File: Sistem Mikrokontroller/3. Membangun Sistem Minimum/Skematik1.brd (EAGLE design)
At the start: 59.4 x 57.1 mm, 20 parts, among them IC2 78L05Z, J1 DCJ0202, U1 328P

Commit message: update
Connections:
- removed net N$37: C3.2, C7.-, S2.2
- net GND: now also C3.2, C7.-, S2.2
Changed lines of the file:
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@@
 <contactref element="JP5" pad="3"/>
 <contactref element="JP5" pad="2"/>
-<wire x1="55.88" y1="41.91" x2="53.34" y2="52.07" width="0" layer="19" extent="1-1"/>
+<contactref element="C3" pad="2"/>
+<contactref element="C7" pad="-"/>
+<contactref element="S2" pad="2"/>
+<wire x1="55.88" y1="41.91" x2="68.58" y2="39.37" width="0" layer="19" extent="1-1"/>
 <wire x1="52.07" y1="40.64" x2="55.88" y2="41.91" width="0" layer="19" extent="16-16"/>
 <wire x1="41.275" y1="34.925" x2="50.8" y2="34.925" width="0" layer="19" extent="16-16"/>
 <wire x1="36.83" y1="27.94" x2="41.275" y2="34.925" width="0" layer="19" extent="16-16"/>
+<wire x1="53.34" y1="52.07" x2="55.88" y2="41.91" width="0" layer="19" extent="1-1"/>
 <wire x1="13.69" y1="22.86" x2="36.83" y2="27.94" width="0" layer="19" extent="1-1"/>
 <wire x1="8.89" y1="19.86" x2="13.69" y2="22.86" width="0" layer="19" extent="1-1"/>
@@
 <wire x1="17.78" y1="1.27" x2="15.24" y2="1.27" width="0" layer="19" extent="1-1"/>
 <wire x1="10.16" y1="-17.78" x2="10.16" y2="1.27" width="0" layer="19" extent="1-1"/>
-<wire x1="8.89" y1="-48.26" x2="10.16" y2="-17.78" width="0" layer="19" extent="1-1"/>
+<wire x1="10.16" y1="-34.29" x2="10.16" y2="-17.78" width="0" layer="19" extent="1-1"/>
+<wire x1="-1.5494" y1="-31.7246" x2="10.16" y2="-34.29" width="0" layer="19" extent="1-1"/>
+<wire x1="8.89" y1="-48.26" x2="10.16" y2="-34.29" width="0" layer="19" extent="1-1"/>
 <wire x1="6.35" y1="-48.26" x2="8.89" y2="-48.26" width="0" layer="19" extent="1-1"/>
 <wire x1="3.81" y1="-48.26" x2="6.35" y2="-48.26" width="0" layer="19" extent="1-1"/>
@@
 <wire x1="16.51" y1="-41.91" x2="13.97" y2="-41.91" width="0" layer="19" extent="1-1"/>
 </signal>
-<signal name="N$37">
-<contactref element="C3" pad="2"/>
-<contactref element="C7" pad="-"/>
-<contactref element="S2" pad="2"/>
-<wire x1="10.16" y1="-34.29" x2="68.58" y2="39.37" width="0" layer="19" extent="1-1"/>
-<wire x1="-1.5494" y1="-31.7246" x2="10.16" y2="-34.29" width="0" layer="19" extent="1-1"/>
-</signal>
 <signal name="N$38">

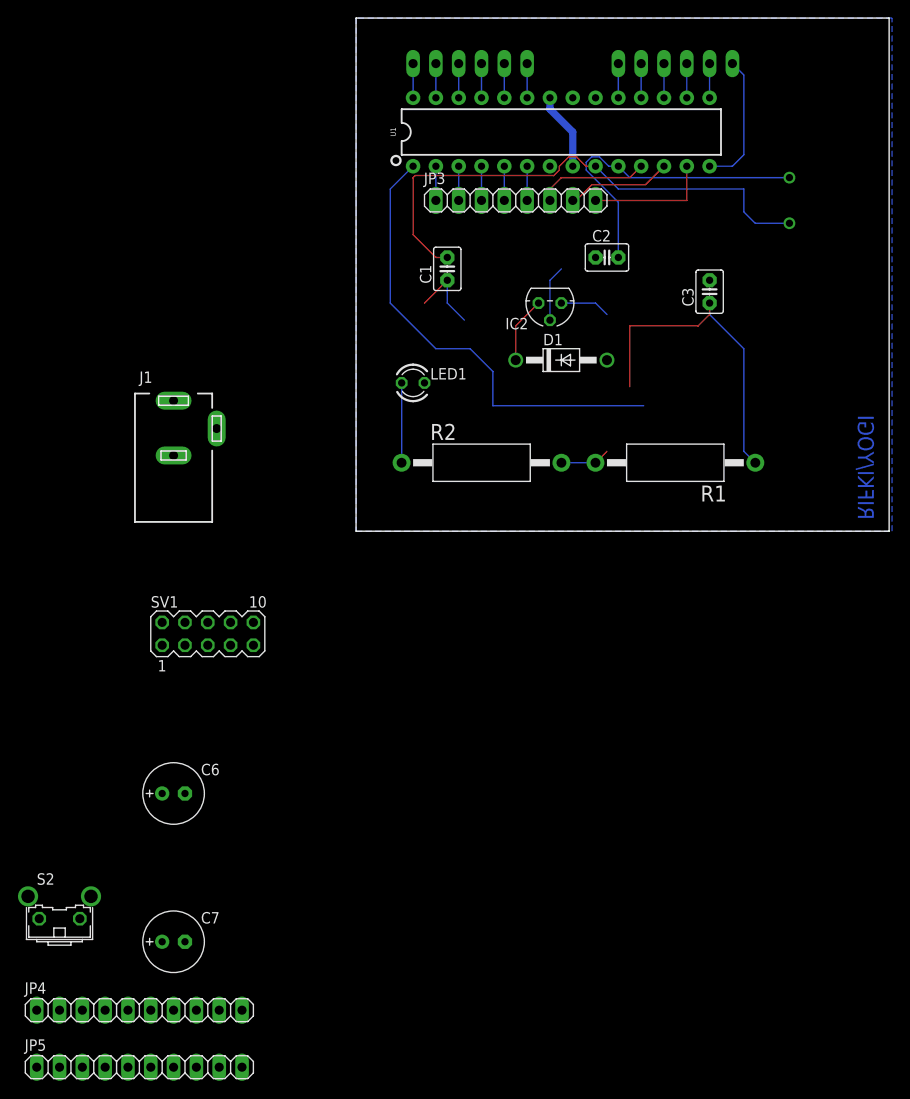
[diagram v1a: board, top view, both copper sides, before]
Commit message: update
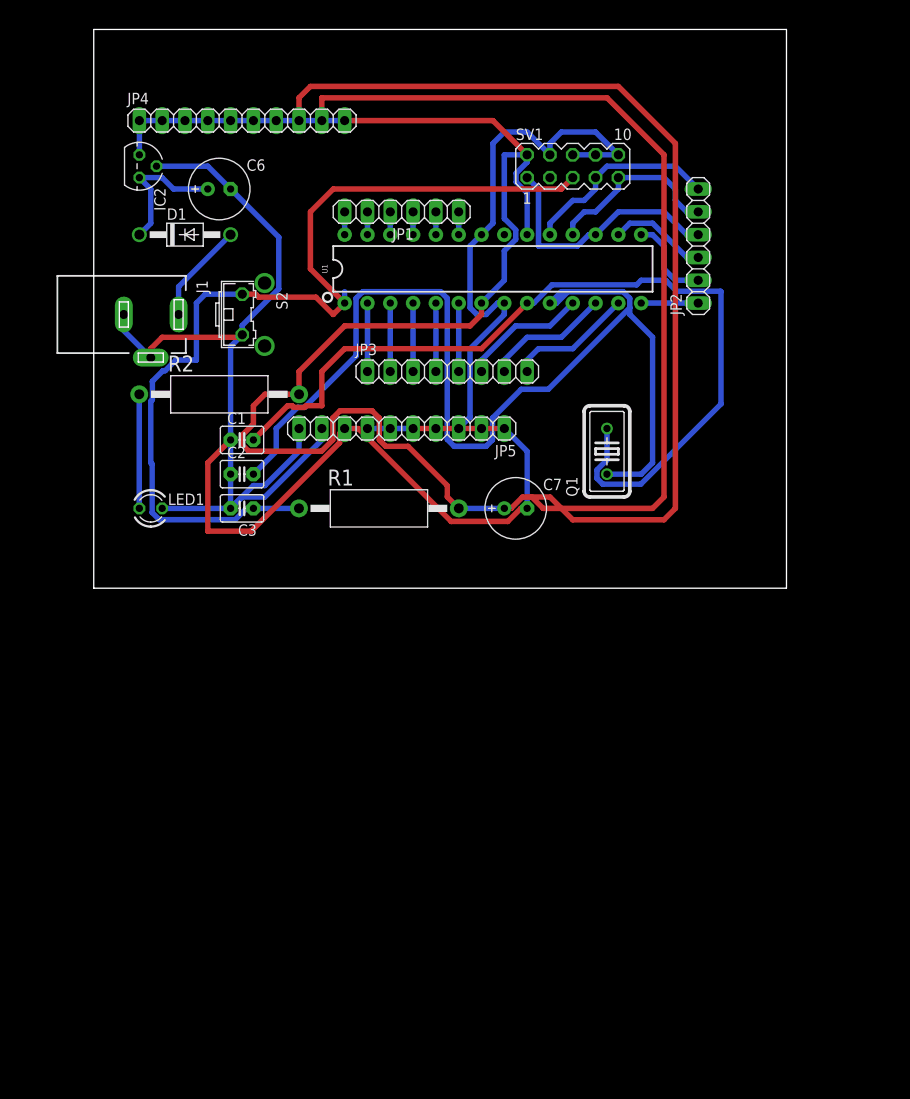
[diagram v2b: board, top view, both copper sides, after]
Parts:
- moved JP4 99.7 mm to (16.5, 57.1)
- moved JP5 76.9 mm to (34.3, 22.9), turned to 180 degrees
- moved S2 69.5 mm to (17.8, 35.6), turned to 270 degrees
- moved C6 67.5 mm to (14.0, 49.5)
- moved SV1 66.1 mm to (53.3, 52.1)
- moved C7 61.5 mm to (47.0, 14.0)
- moved C3 57.4 mm to (16.5, 14.0), turned to 180 degrees
- moved IC2 48.2 mm to (5.08, 52.1), turned to 270 degrees
- moved C2 47.3 mm to (16.5, 17.8)
- moved D1 44.2 mm to (10.2, 44.5)
- moved Q1 34.5 mm to (57.1, 20.3), flipped to the top, turned to 90 degrees
- moved R1 33.4 mm to (31.8, 14.0), turned to 0 degrees
- moved LED1 32.4 mm to (6.35, 14.0)
- moved R2 30.2 mm to (14.0, 26.7)
- moved C1 29.8 mm to (16.5, 21.6), turned to 0 degrees
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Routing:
- net VCC: track 11.2 -> 362.8 mm
- net GND: track 23.7 -> 247.9 mm
- net N$3: track 35.9 -> 116.9 mm
- net N$2: track 58.9 -> 98.6 mm
- net N$28: track 3.81 -> 28.6 mm
- net N$30: track 3.81 -> 22.2 mm
- net N$34: track 88.8 -> 106.4 mm
- net N$29: track 3.81 -> 20.4 mm
- net N$21: track 0.00 -> 11.3 mm
- net N$25: track 15.0 -> 6.35 mm
- net N$38: track 7.40 -> 15.5 mm
- net N$27: track 3.81 -> 11.0 mm
- net N$26: track 3.81 -> 9.94 mm
- net N$36: track 8.89 -> 12.7 mm
- net N$9: track 3.81 -> 7.62 mm
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- removed copper zone on layer 16, net RY
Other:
- board size 59.4 x 57.1 mm -> 77.1 x 62.2 mm
- board text removed: "RIFKI/YOGI"
